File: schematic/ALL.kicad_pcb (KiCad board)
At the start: 4 copper layers, 200 x 80 mm, 126 parts, among them CON1 USB-MICRO-B

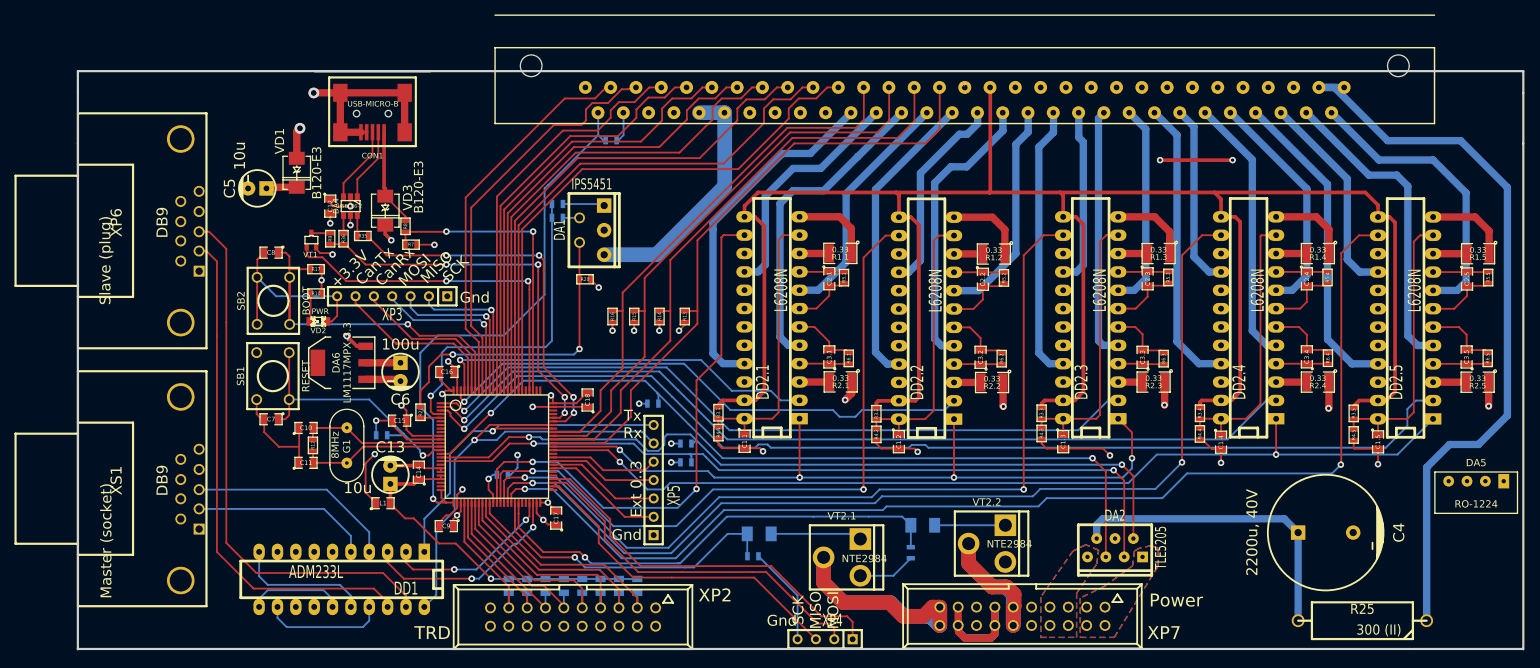
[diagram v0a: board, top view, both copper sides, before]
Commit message: modified schematics
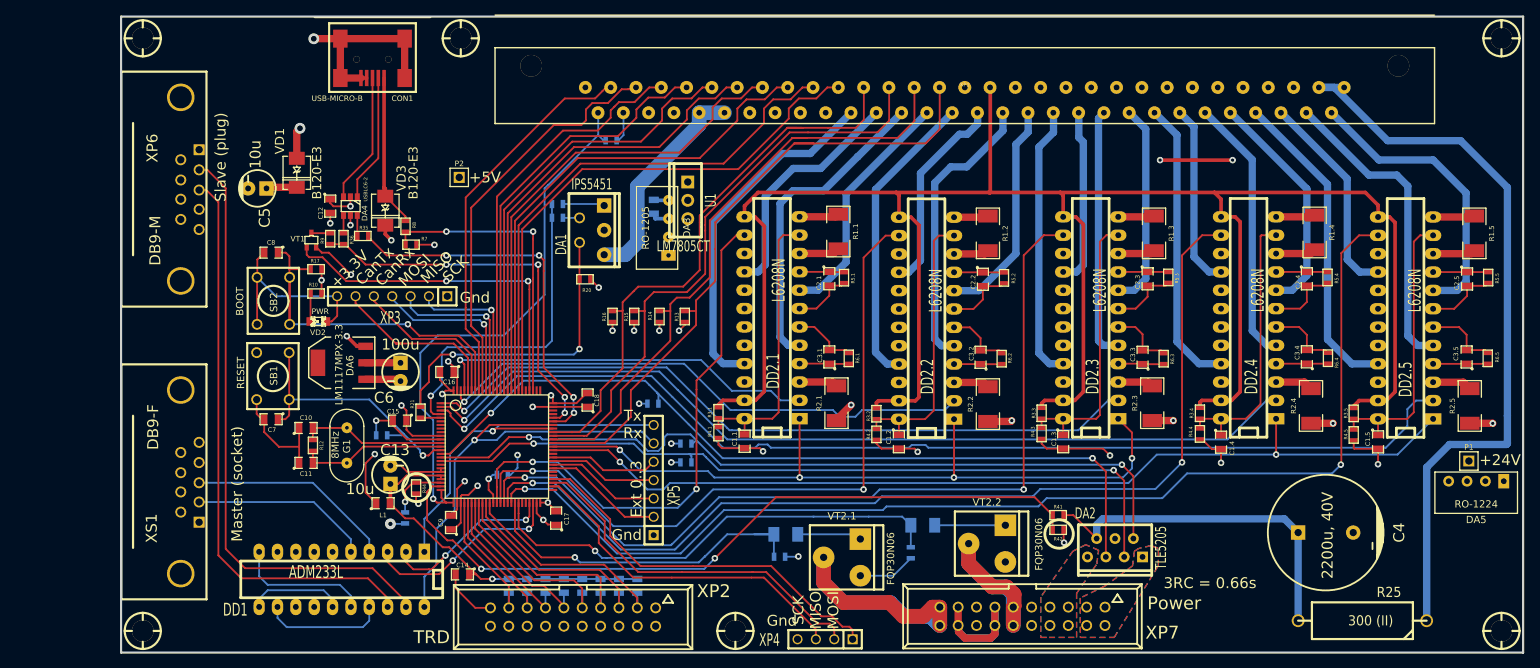
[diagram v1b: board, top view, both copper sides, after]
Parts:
- added C19: 1u, SM0805, B.Cu at (124.7, 83.3)
- added DA3: RO-1205, SIP-4-RO, F.Cu at (126.7, 86.2)
- added HOLE1: 3mm, hole_3mm, F.Cu at (54.0, 142.0)
- added HOLE2: 3mm, hole_3mm, F.Cu at (54.0, 60.0)
- added HOLE3: 3mm, hole_3mm, F.Cu at (242.0, 142.0)
- added HOLE4: 3mm, hole_3mm, F.Cu at (136.0, 142.0)
- added HOLE5: 3mm, hole_3mm, F.Cu at (242.0, 60.0)
- added HOLE6: 3mm, hole_3mm, F.Cu at (98.0, 60.0)
- added P1: CONN_1, PIN_ARRAY_1, F.Cu at (237.5, 118.5)
- added P2: CONN_1, PIN_ARRAY_1, F.Cu at (97.8, 79.2)
- added R41: 56k, SM0603, F.Cu at (180.7, 126.0)
- added R42: 4.7k, SM0603, F.Cu at (180.7, 128.0)
- added R43: 12k, SM0603, B.Cu at (90.3, 126.4)
- added R44: 4.7k, SM0603, F.Cu at (91.8, 122.2)
- added U1: LM7805CT, TO220_VERT, F.Cu at (129.4, 82.4)
- R1.1, R1.2, R1.3, R1.4, R1.5, R2.1, R2.2, R2.3, R2.4, R2.5: footprint SM1210 -> SM-2010
- VT2.1, VT2.2: value NTE2984 -> FQP30N06
- XP6: value DB9 -> DB9-M; footprint DB9FC -> DB9-M
- XS1: value DB9 -> DB9-F; footprint DB9FC -> DB9-F
- moved C14 15.4 mm to (98.2, 134.2), turned to 180 degrees
- moved CON1 7.50 mm to (85.8, 62.9)
- moved XP6 5.77 mm to (60.5, 81.0)
- moved R38 3.68 mm to (142.1, 131.7)
- moved R40.1 3.68 mm to (143.0, 128.6)
- moved R2.5 3.46 mm to (237.6, 110.9), turned to 90 degrees
- moved R2.4 3.44 mm to (215.6, 110.9), turned to 90 degrees
- moved R2.2 3.04 mm to (170.9, 110.6), turned to 90 degrees
- moved R1.1 3.04 mm to (150.2, 86.7), turned to 270 degrees
- moved R2.1 3.00 mm to (150.0, 110.5), turned to 90 degrees
- moved R1.2 2.97 mm to (170.9, 87.0), turned to 270 degrees
- moved R1.4 2.95 mm to (216.2, 86.9), turned to 270 degrees
- moved R2.3 2.93 mm to (193.7, 110.5), turned to 90 degrees
- moved R1.3 2.87 mm to (193.9, 87.0), turned to 270 degrees
- moved R1.5 2.86 mm to (238.3, 87.0), turned to 270 degrees
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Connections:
- DA5 pad 1: /Filters slit #1/+10V -> GND
- DA5 pad 2: GND -> /Filters slit #1/+10V
- DA5 pad 3: /Filters slit #1/+24V -> GND
- DA5 pad 4: GND -> /Filters slit #1/+24V
- DD1 pad 18: N-00000157 -> N-00000155
- DD3 pad 23: (no net) -> /STM32F103 module/U10
- DD3 pad 24: (no net) -> /Shutter MOSFET/Sense
- VT1 pad 2: +5V -> +3.3V
- XP6 pad 2: N-00000157 -> N-00000169
- XP6 pad 3: N-00000169 -> N-00000155
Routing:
- net /Shutter MOSFET/Sense: track 0.00 -> 102.7 mm, vias 0 -> 2
- net N-00000155: track 0.00 -> 79.3 mm
- net /Filters slit #1/+10V: track 41.4 -> 119.7 mm, vias 0 -> 1
- net +5V: track 381.6 -> 453.3 mm, vias 5 -> 4
- net N-00000157: track 70.4 -> 0.00 mm
- net (no net): track 57.0 -> 0.00 mm
- net GND: track 338.9 -> 309.3 mm, vias 20 -> 23
- net +3.3V: track 100.1 -> 111.7 mm, vias 14 -> 15
- net N-00000175: track 13.5 -> 22.2 mm
- net N-00000169: track 74.9 -> 83.3 mm
- net /STM32F103 module/U10: track 0.00 -> 8.46 mm, vias 0 -> 1
- net N-00000171: track 10.2 -> 17.7 mm
- net N-00000170: track 10.6 -> 18.1 mm
- net /EP3: track 74.6 -> 81.7 mm
- net N-00000147: track 43.1 -> 49.0 mm
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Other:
- board size 200 x 80 mm -> 194 x 88 mm
- board text added: "+24V"
- board text added: "+5V"
- board text added: "3RC = 0.66s"
